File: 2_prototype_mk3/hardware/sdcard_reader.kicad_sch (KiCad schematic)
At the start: 4 parts, among them J1 Micro_SD_Card

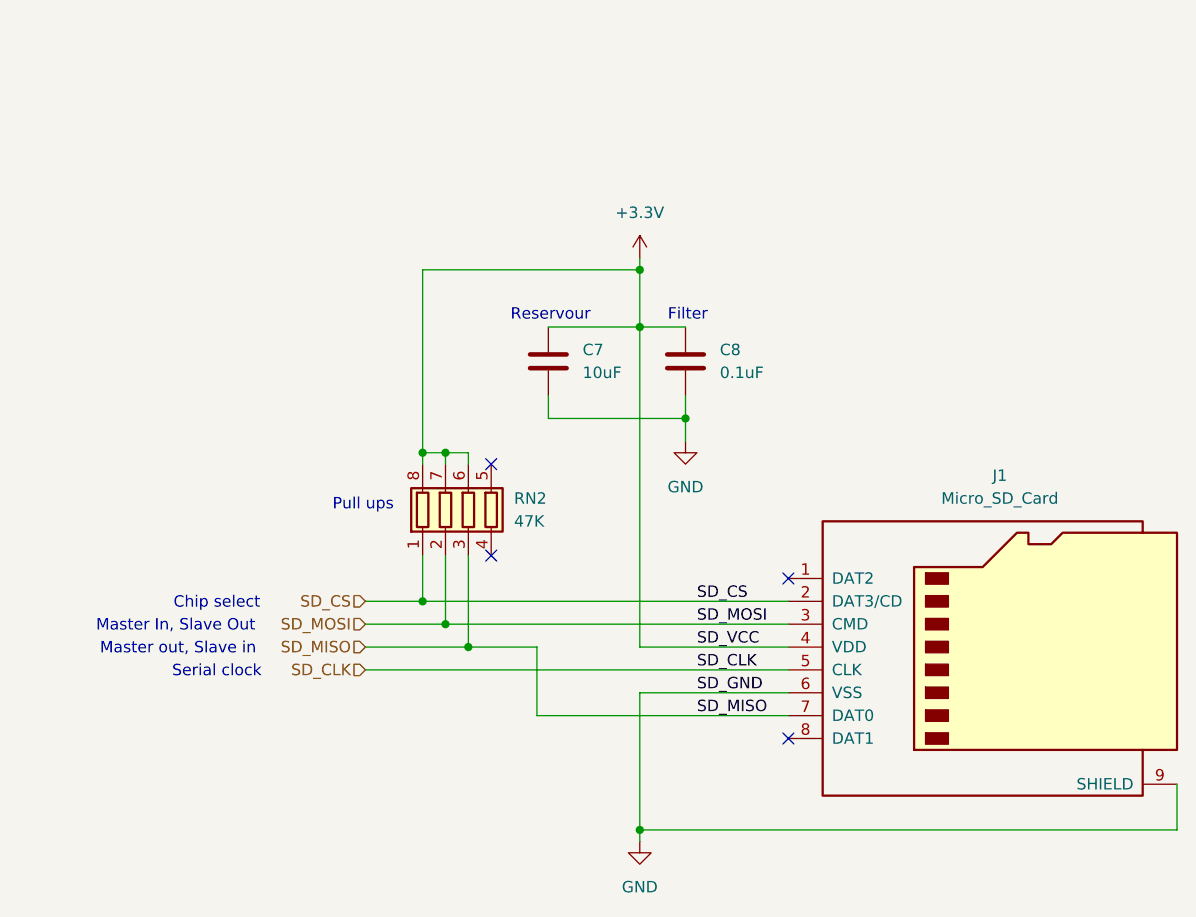
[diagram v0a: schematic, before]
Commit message: MKIII design refinements
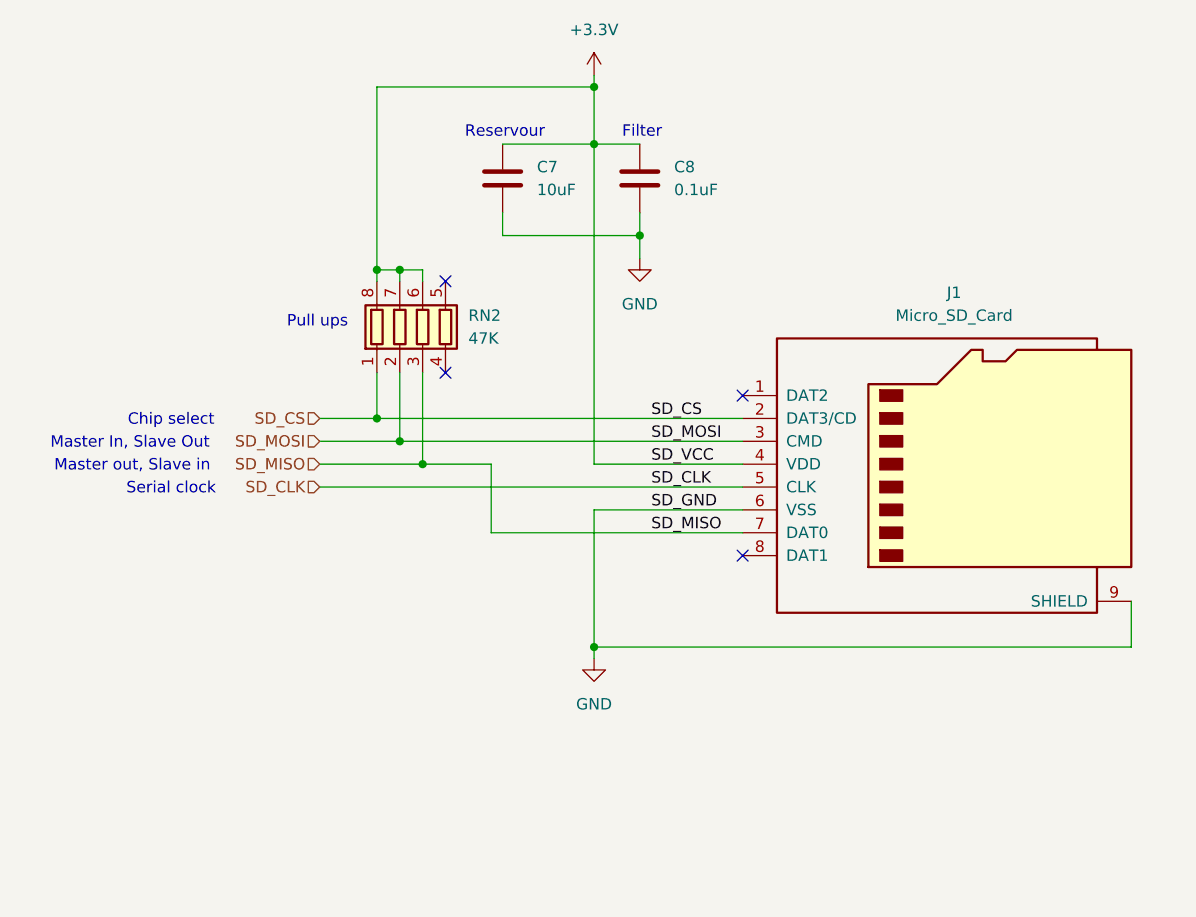
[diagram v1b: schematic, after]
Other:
- title: (none) -> SD card reader
- moved on the sheet: C7, C8, J1, RN2
